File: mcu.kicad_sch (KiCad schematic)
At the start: 5 parts, among them J3 USB_C_Receptacle_USB2.0_16P, M1 Module-stlink-0.1, M3 Module-mega-mcu144-0.6

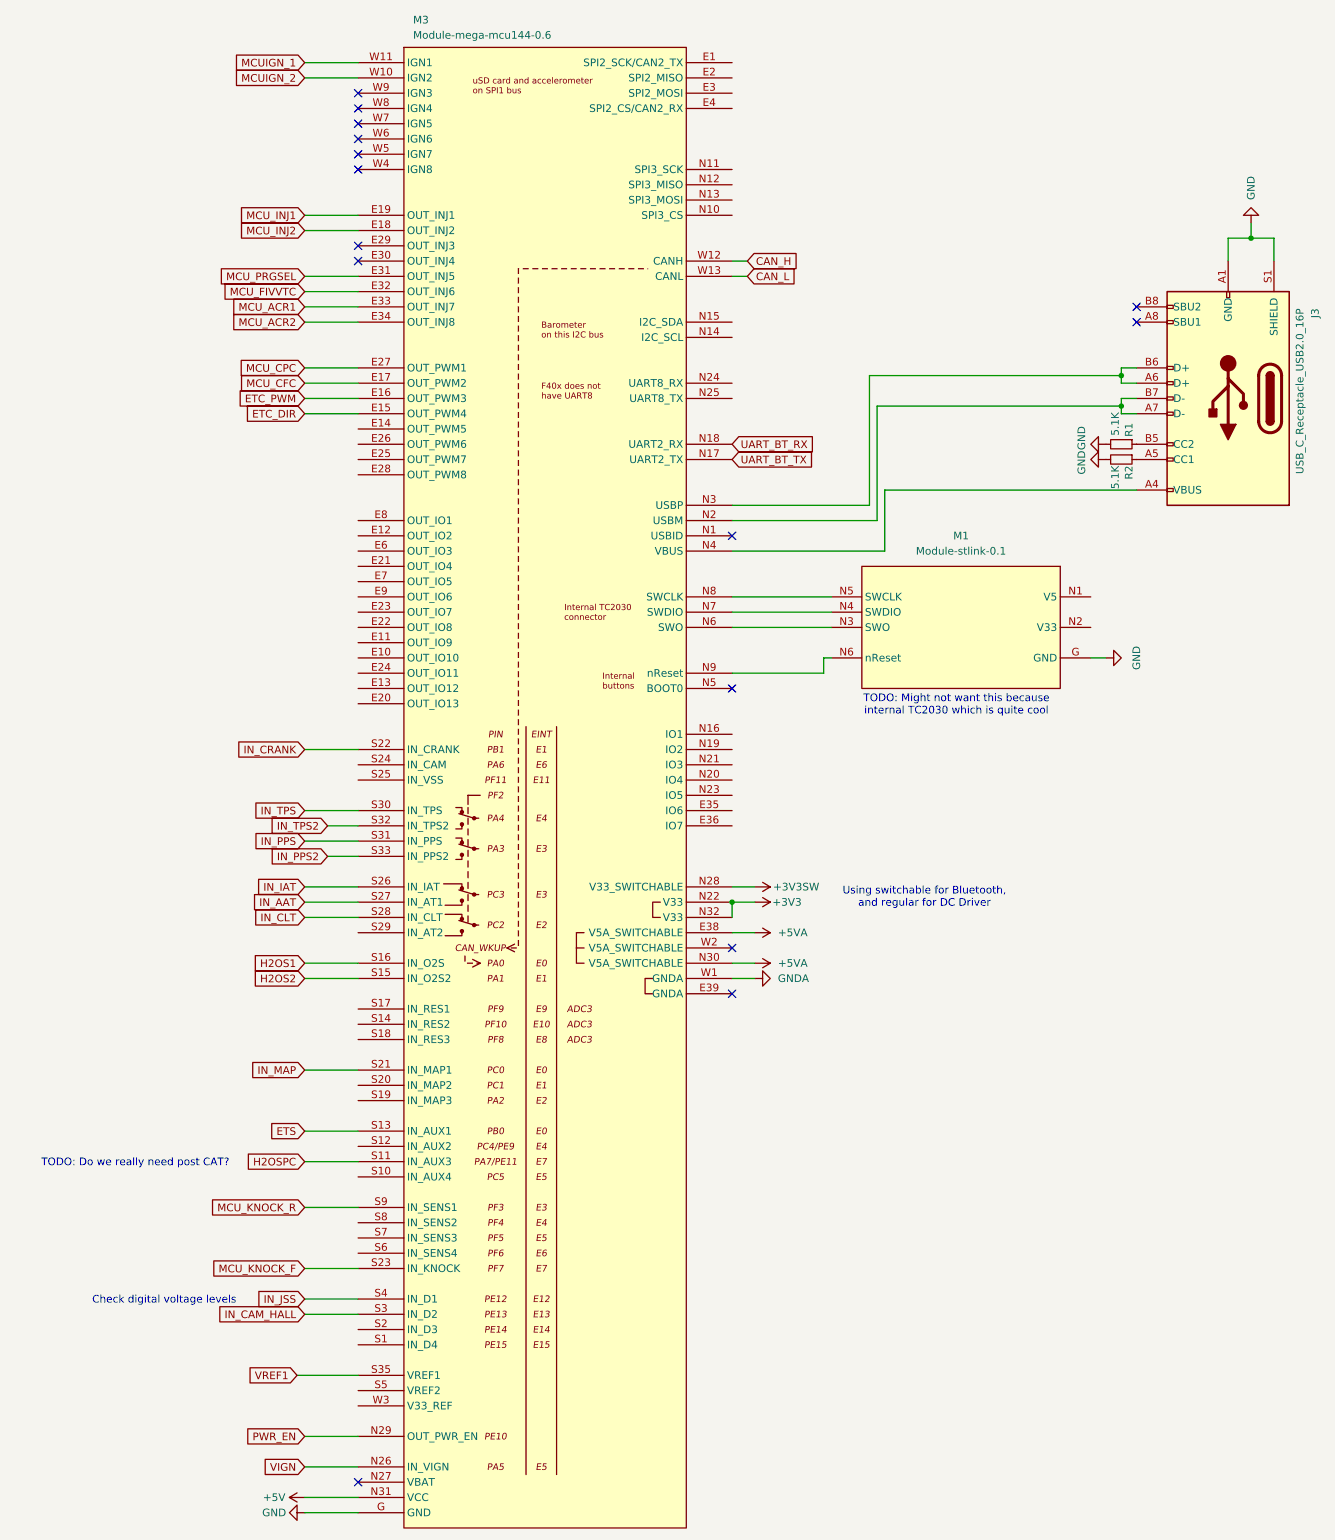
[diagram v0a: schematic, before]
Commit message: redone layout, possibly feature complete
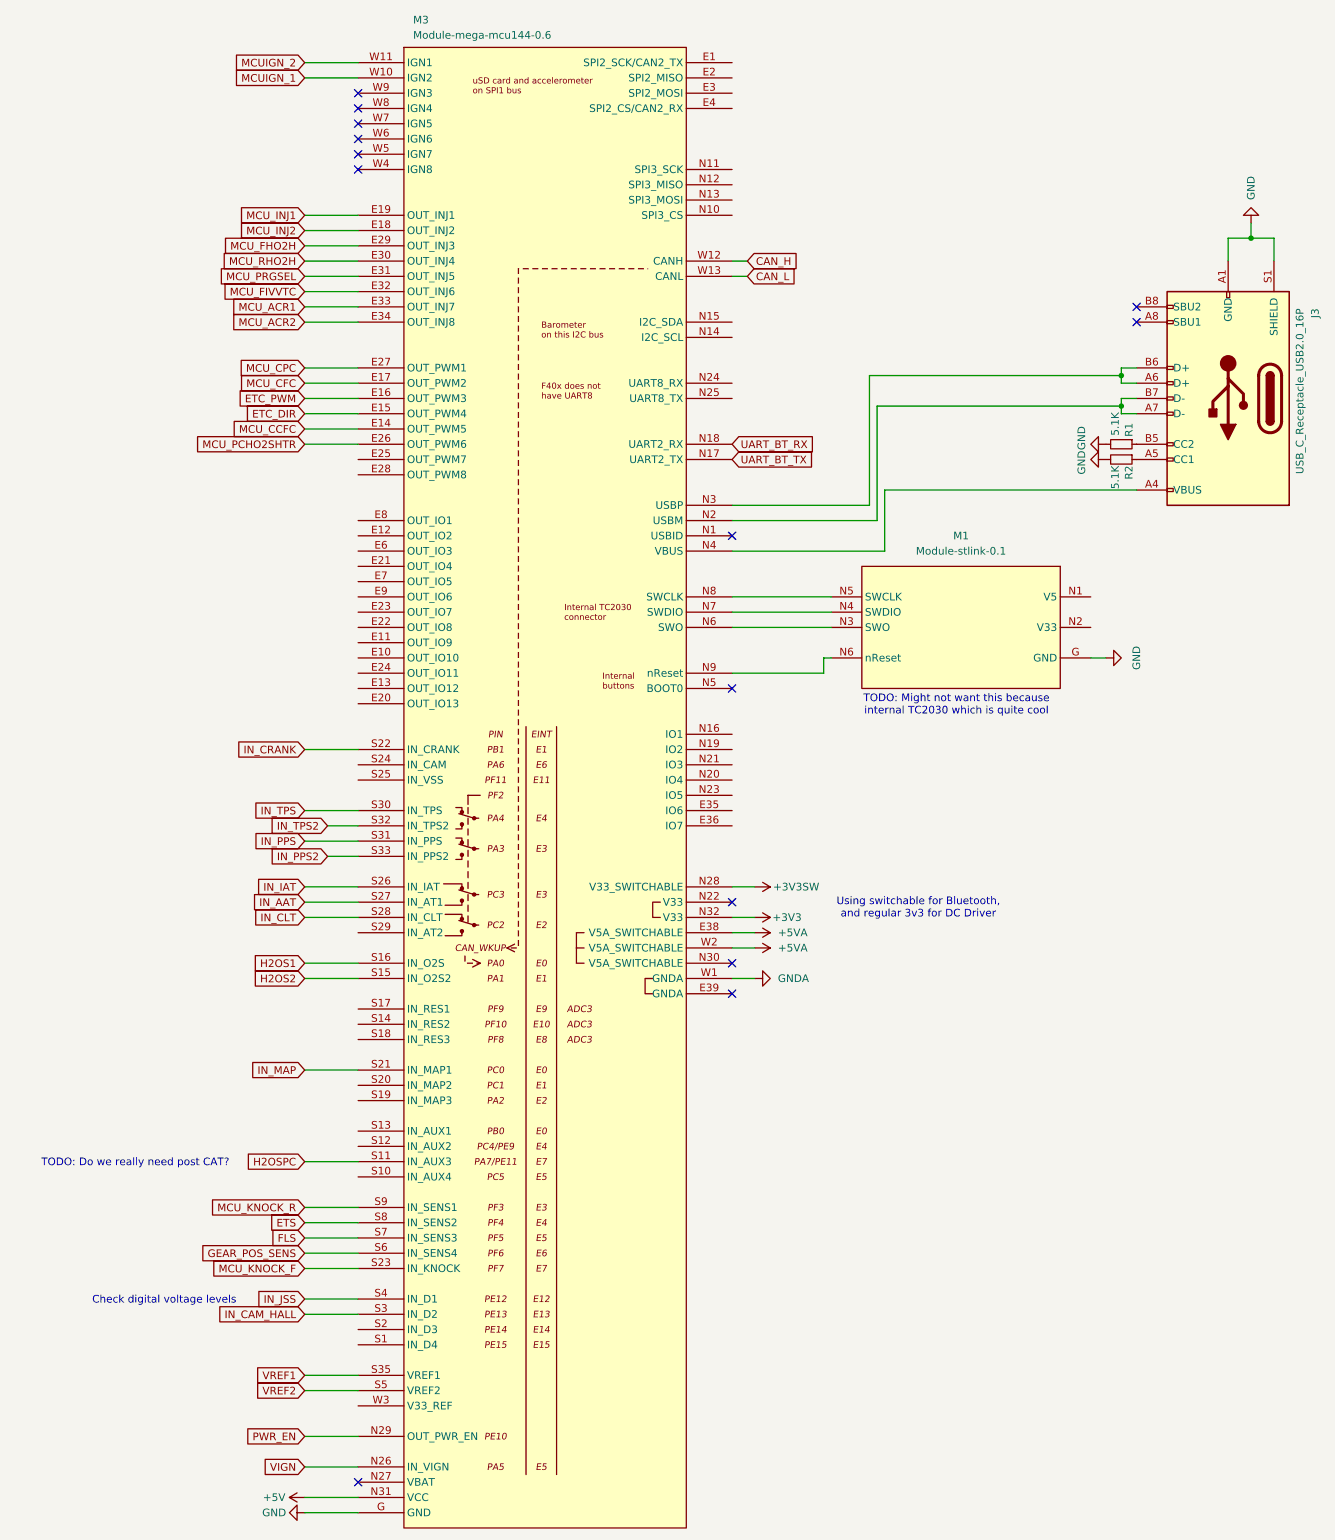
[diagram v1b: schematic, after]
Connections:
- net +3V3: no longer M3.N22 (V33)
- net +5VA: now also M3.W2 (V5A_SWITCHABLE); no longer M3.N30 (V5A_SWITCHABLE)
- net ETS: now also M3.S8 (IN_SENS2); no longer M3.S13 (IN_AUX1)
- net MCUIGN_1: now also M3.W10 (IGN2); no longer M3.W11 (IGN1)
- net MCUIGN_2: now also M3.W11 (IGN1); no longer M3.W10 (IGN2)
- net MCU_CCFC: now reaches M3.E14 (OUT_PWM5)
- net MCU_PCHO2SHTR: now reaches M3.E26 (OUT_PWM6)
- net MCU_FHO2H: now reaches M3.E29 (OUT_INJ3)
- net MCU_RHO2H: now reaches M3.E30 (OUT_INJ4)
- net VREF2: now reaches M3.S5 (VREF2)
- net GEAR_POS_SENS: now reaches M3.S6 (IN_SENS4)
- net FLS: now reaches M3.S7 (IN_SENS3)
- no-connect marks 15 -> 14
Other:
- note added: "Using switchable for Bluetooth, and regular 3v3 for DC Driver"
- note removed: "Using switchable for Bluetooth, and regular for DC Driver"
